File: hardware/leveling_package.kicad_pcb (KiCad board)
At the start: 2 copper layers, 100 x 100 mm, 20 parts, among them J1 Conn_01x16_Male, J2 Conn_01x16_Male, J3 Conn_01x16_Male, J4 Conn_01x16_Male, Q1 BSS138, SW1 SW_Push

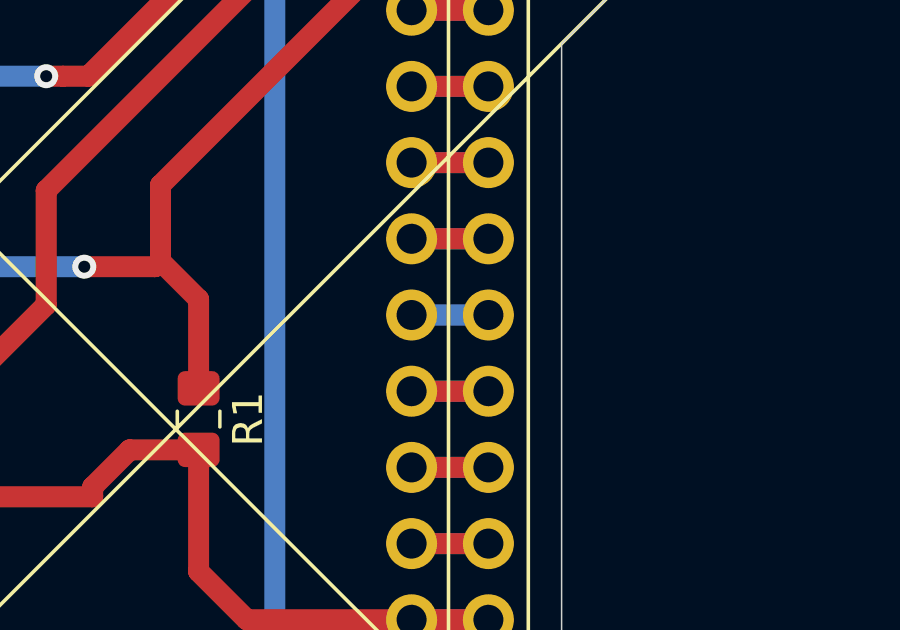
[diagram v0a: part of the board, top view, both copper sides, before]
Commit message: trig functions started
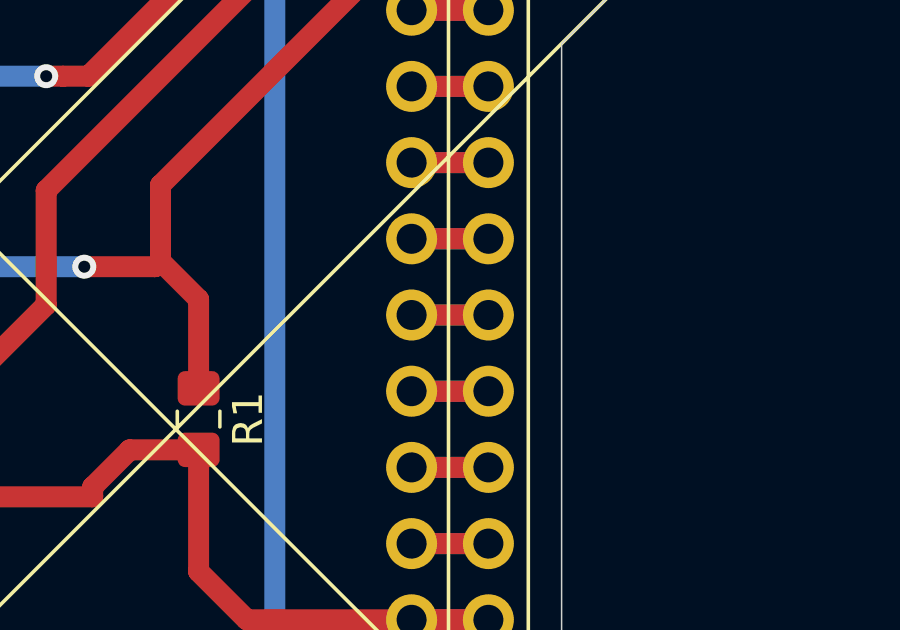
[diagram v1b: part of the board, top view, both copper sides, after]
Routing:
- net Net-(J1-Pad7): track 2.56 -> 5.12 mm
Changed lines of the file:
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@@
     (thickness 1.6)
     (drawings 29)
-    (tracks 329)
+    (tracks 330)
     (zones 0)
     (modules 20)
@@
     (visible_elements FFFFFF7F)
     (pcbplotparams
-      (layerselection 0x00000_7fffffff)
+      (layerselection 0x01000_7fffffff)
       (usegerberextensions false)
       (usegerberattributes false)
@@
   (segment (start 96 72.73) (end 98.56 72.73) (width 0.7) (layer B.Cu) (net 9))
   (segment (start 98.56 70.19) (end 96 70.19) (width 0.7) (layer B.Cu) (net 10))
+  (segment (start 96 70.19) (end 98.56 70.19) (width 0.7) (layer F.Cu) (net 10))
   (segment (start 96 67.65) (end 98.56 67.65) (width 0.7) (layer F.Cu) (net 11))
   (segment (start 96 67.65) (end 98.56 67.65) (width 0.7) (layer B.Cu) (net 11))
@@
       )
     )
+  )
+  (zone (net 0) (net_name "") (layer F.Cu) (hatch edge 0.508)
+    (connect_pads (clearance 0.508))
+    (min_thickness 0.254)
+    (keepout (tracks allowed) (vias allowed) (copperpour not_allowed))
+    (fill (arc_segments 32) (thermal_gap 0.508) (thermal_bridge_width 0.508))
+    (polygon
+      (pts
+        (xy 79.375 78.105) (xy 68.58 78.105) (xy 68.58 68.58) (xy 79.375 68.58)
+      )
+    )
